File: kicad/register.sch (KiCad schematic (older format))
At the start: 11 parts, among them U7 74LS173, U8 74LS173, U9 74LS245

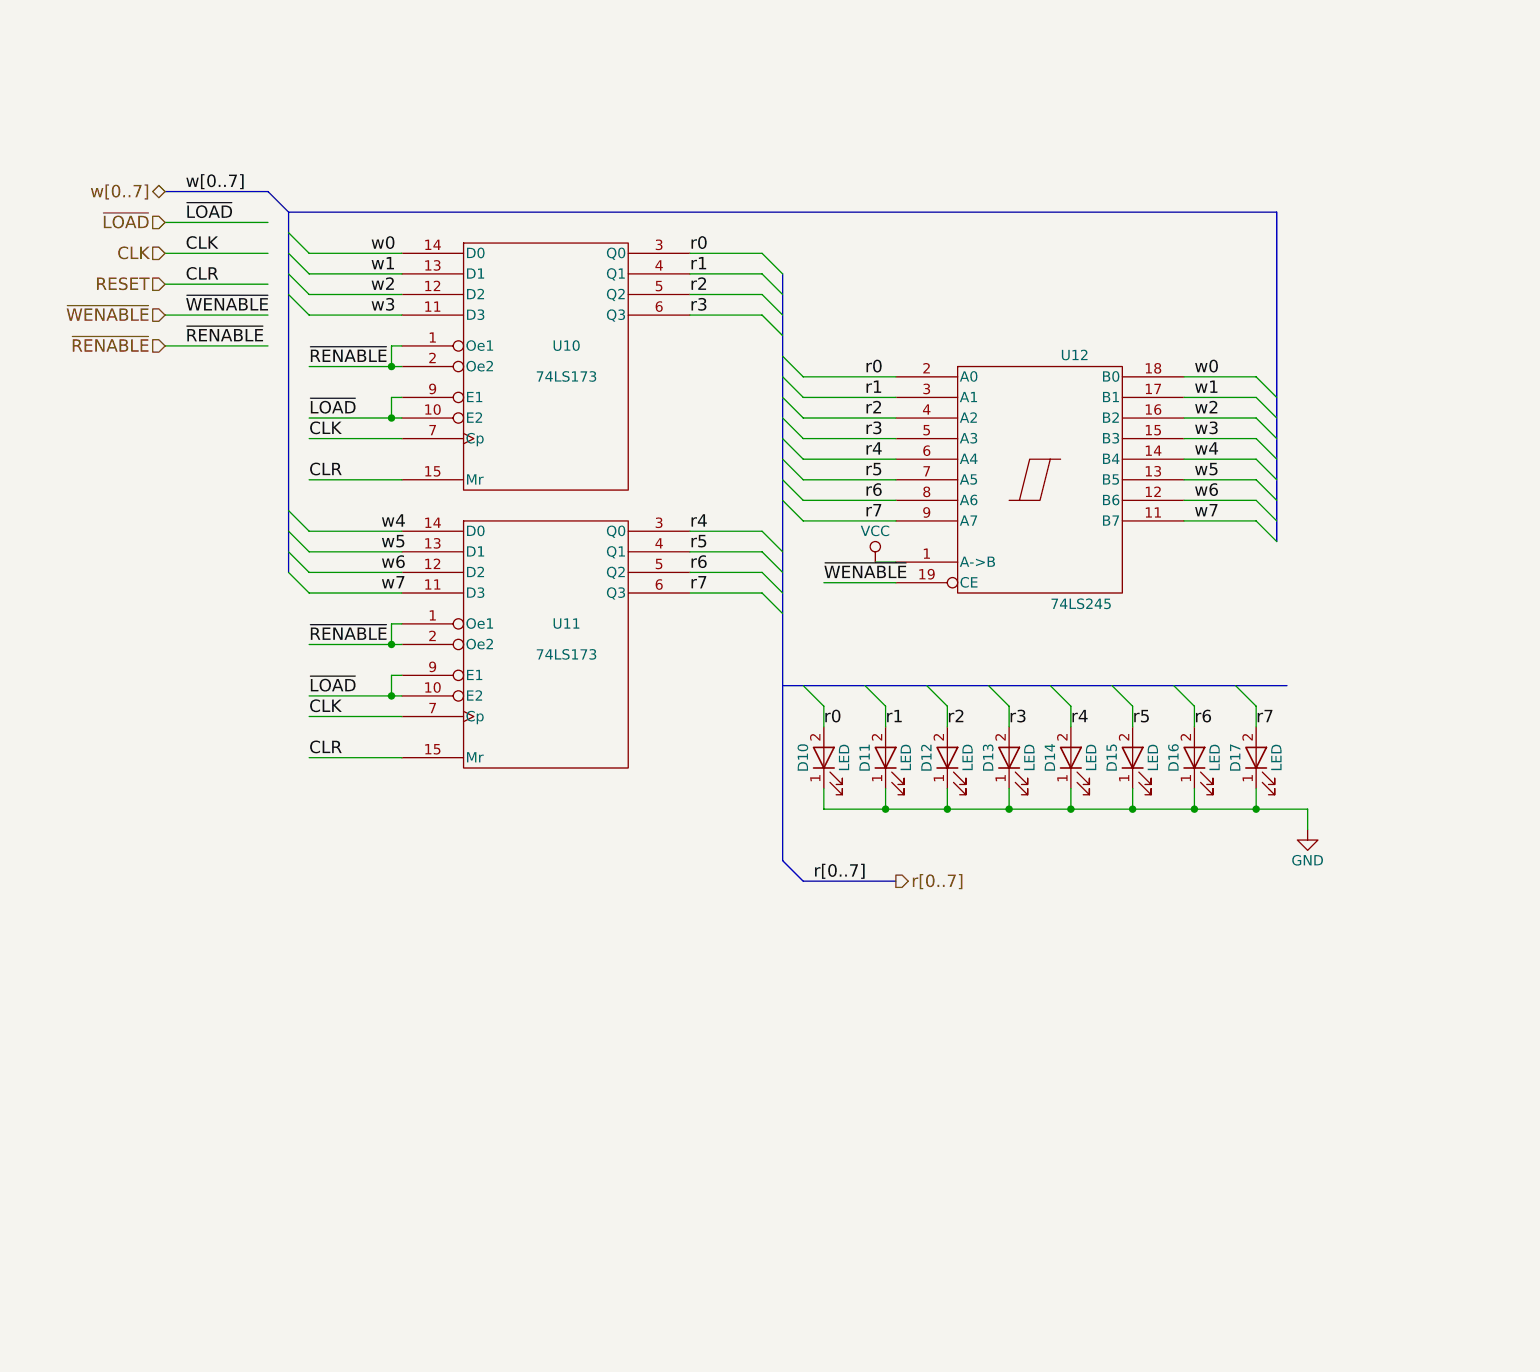
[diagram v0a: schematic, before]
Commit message: Update to current kicad libraries
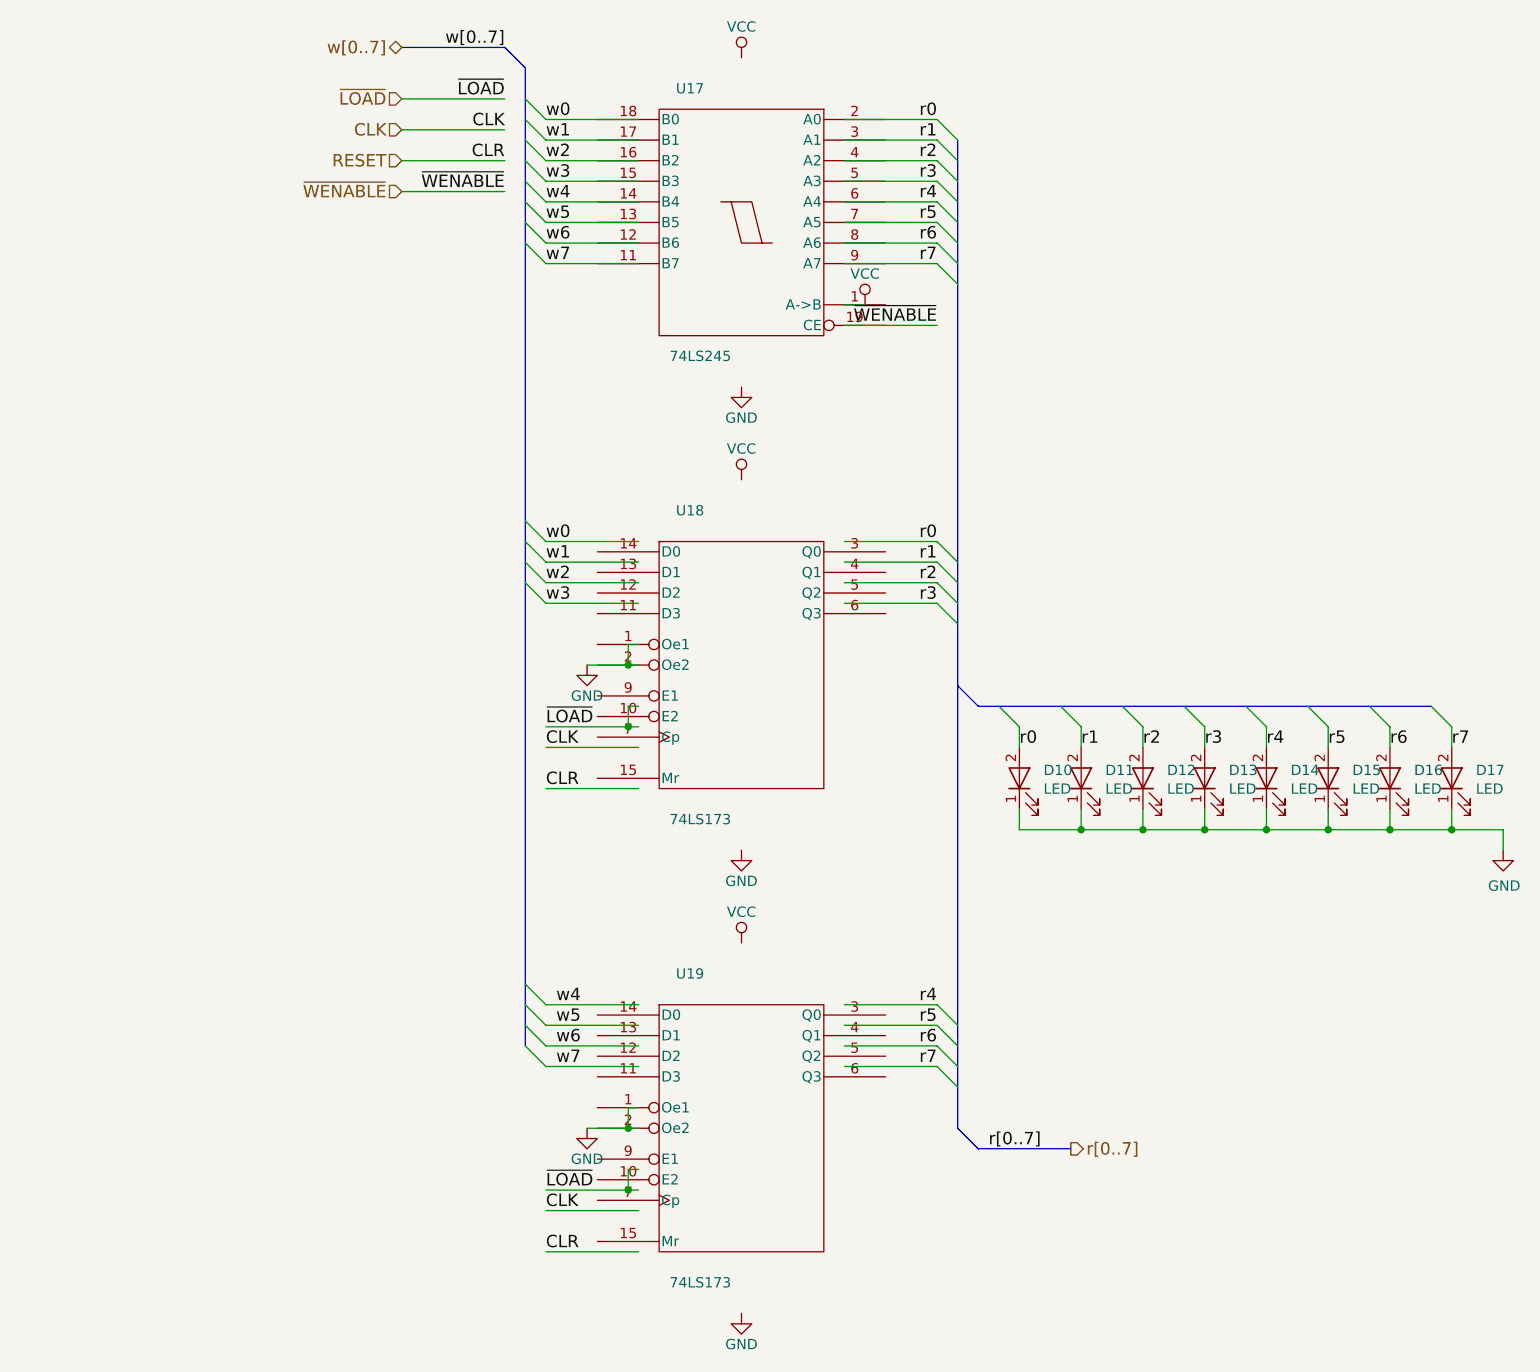
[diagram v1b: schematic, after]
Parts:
- removed D2, D3, D4, D5, D6, D7, D8, D9: LED, LEDs:LED-5MM, symbol LED
- removed U7, U8: 74LS173, Housings_DIP:DIP-16_W7.62mm_LongPads, symbol 74LS173
- removed U9: 74LS245, Housings_DIP:DIP-20_W7.62mm_LongPads, symbol 74LS245
- added D10, D11, D12, D13, D14, D15, D16, D17: LED, symbol Device:LED
- added U17: 74LS245, symbol 74xx:74LS245
- added U18, U19: 74LS173, symbol 74xx:74LS173
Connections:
- net labels removed: ~RENABLE
- wire segments 73 -> 83
